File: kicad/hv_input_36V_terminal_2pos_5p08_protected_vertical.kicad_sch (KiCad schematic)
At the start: 15 parts, among them J501 TBH-1x02-5.08mm, U501 TPS1HTC100QPWPRQ1

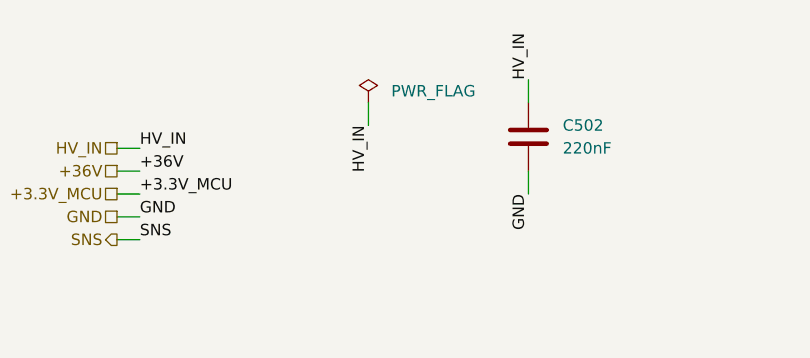
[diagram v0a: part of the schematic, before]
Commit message: Update design rules
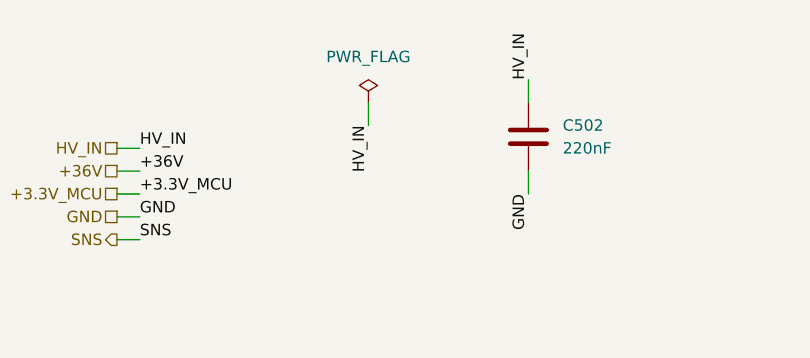
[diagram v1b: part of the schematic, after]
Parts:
- C501: LCSC (none) -> C115056; Vendor SKU (none) -> C115056
- C502: LCSC (none) -> C513710; Vendor SKU (none) -> C513710
- C503: LCSC (none) -> C161234; Vendor SKU (none) -> C161234
- D501: LCSC (none) -> C211388; Vendor SKU (none) -> C211388
- J501: LCSC (none) -> C480503; Vendor SKU (none) -> C480503
- R501, R505: LCSC (none) -> C106235; Vendor SKU (none) -> C106235
- R502, R503, R504, R506, R507: LCSC (none) -> C278577; Vendor SKU (none) -> C278577
- R508: LCSC (none) -> C3016445; Vendor SKU (none) -> C3016445
- R509: LCSC (none) -> C482112; Vendor SKU (none) -> C482112
- U501: LCSC (none) -> C41558366; Vendor SKU (none) -> C41558366
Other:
- company: (none) -> Janelia Research Campus
- title: Orb Weaver Design Block Mining -> mouse-joystick-pcb

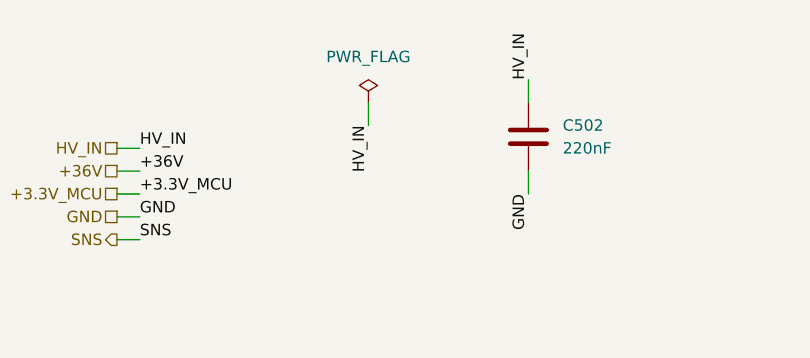
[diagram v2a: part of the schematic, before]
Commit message: Finish v1.0 schematic
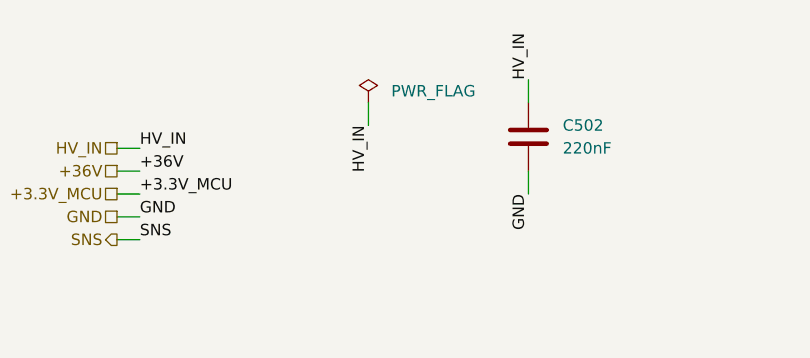
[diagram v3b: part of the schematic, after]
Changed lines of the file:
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@@
 		)
 		(property "Value" "PWR_FLAG"
-			(at 104.14 38.1 0)
+			(at 106.68 41.9099 0)
 			(show_name no)
 			(do_not_autoplace no)
@@
 					(size 1.27 1.27)
 				)
+				(justify left)
 			)
 		)
